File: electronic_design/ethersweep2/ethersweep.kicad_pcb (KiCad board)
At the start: 2 copper layers, 79 x 38 mm, 69 parts, among them J1 AVR-ISP-6, J2 Conn_01x02_Male, J3 Conn_01x04_Female, J4 Conn_01x02_Male, J5 Conn_01x02_Male, J6 HR911105A, J7 Conn_01x06_Female, J8 AVR-ISP-6, J9 Conn_01x06_Male, M1 Stepper_Motor_bipolar, SW1 SW_Push, U1 ENC28J60x-SS, U2 ATmega328-AU, U3 DRV8825PWPR, U4 AMS1117-3.3, U5 AS5600, Y1 Crystal_25MHz, Y2 Crystal_8MHz

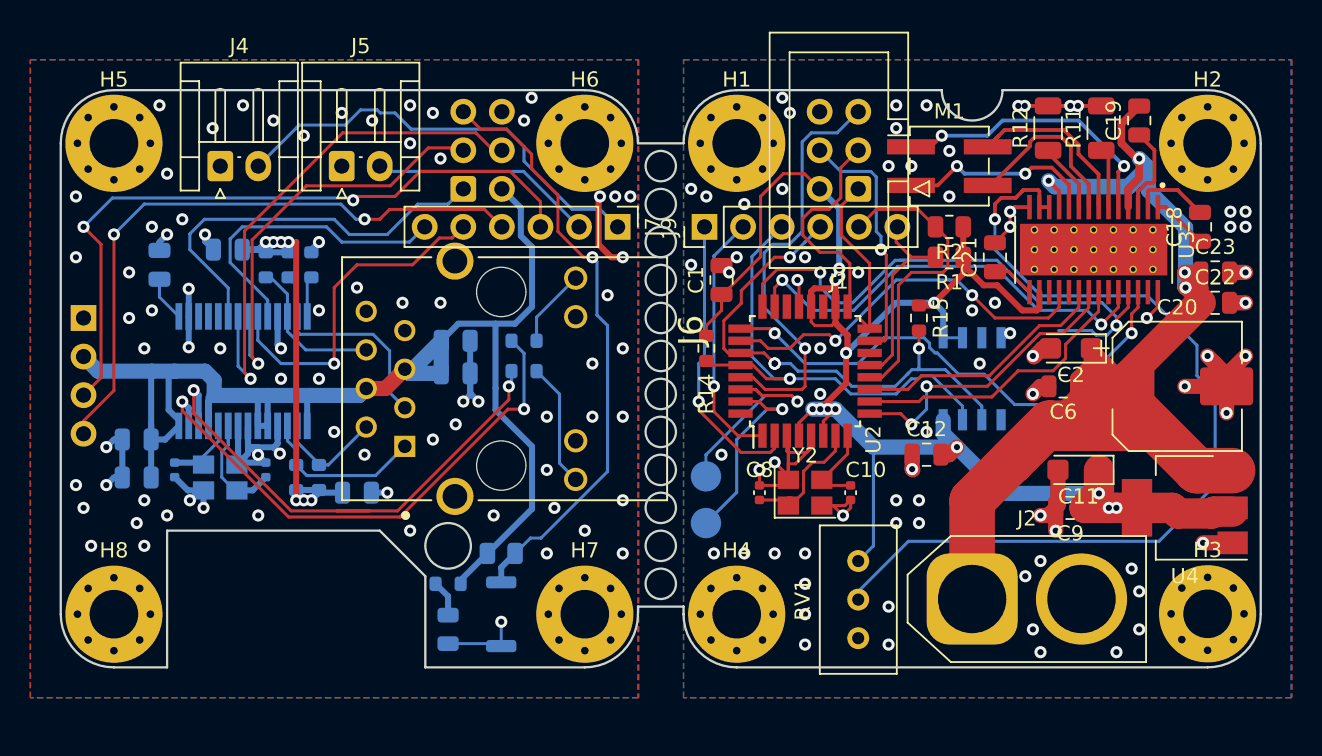
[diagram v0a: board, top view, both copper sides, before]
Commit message: design improvements and error fixes
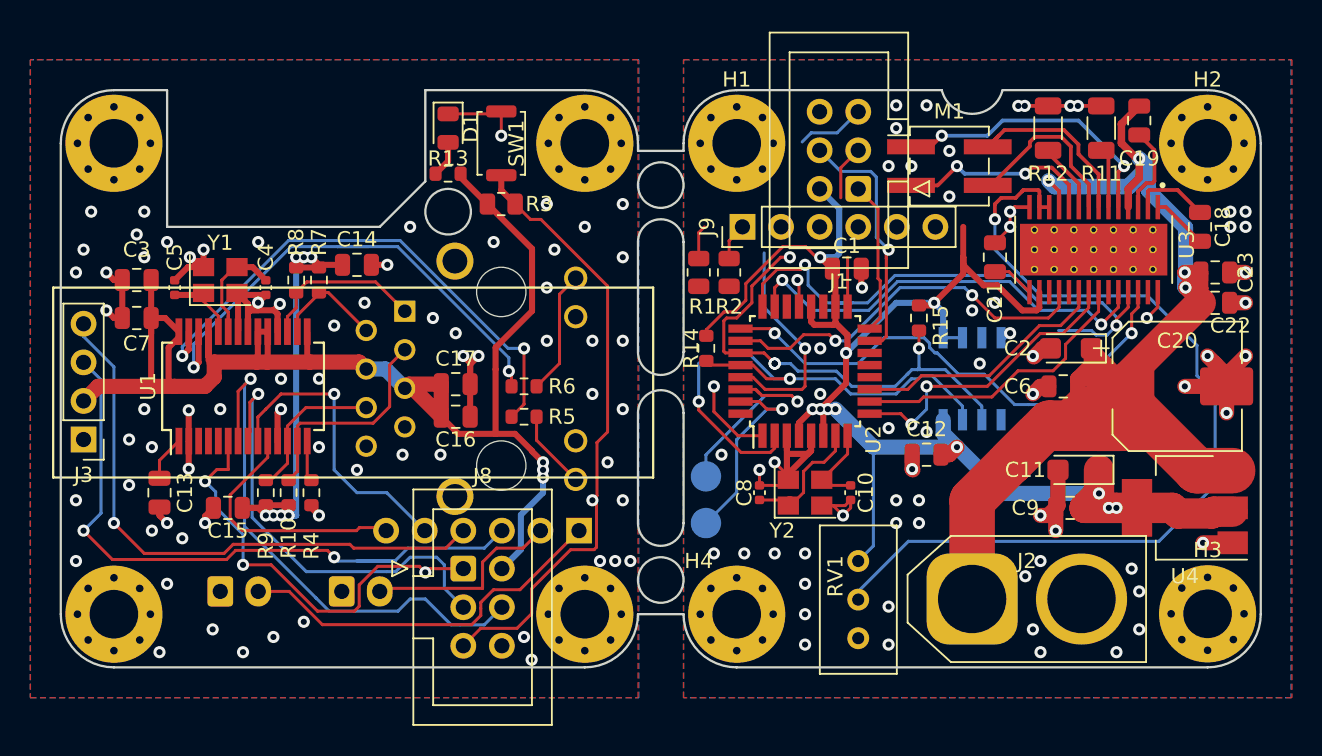
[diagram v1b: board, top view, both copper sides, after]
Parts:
- C13, C14, C15, C16, C17, C3, C4, C5, C7, D1, J3, J8, R10, R13, R3, R4, R5, R6, R7, R8, R9, SW1, U1, Y1: moved to F.Cu
- H5, H6, H7, H8, J4, J5, J6, J7: moved to B.Cu
- moved D1 33.0 mm to (148.0, 83.5), turned to 270 degrees
- moved H5 31.0 mm to (126.0, 115.5)
- moved H6 31.0 mm to (157.0, 115.5)
- moved H7 31.0 mm to (157.0, 84.5)
- moved H8 31.0 mm to (126.0, 84.5)
- moved SW1 31.0 mm to (151.5, 84.5), turned to 90 degrees
- moved J4 28.0 mm to (133.0, 114.0)
- moved J5 28.0 mm to (141.0, 114.0)
- moved R13 27.0 mm to (148.0, 86.5)
- moved J8 25.0 mm to (149.0, 112.5)
- moved R3 23.0 mm to (151.5, 88.5)
- moved J7 20.2 mm to (156.6, 110.0), turned to 90 degrees
- moved C15 17.0 mm to (133.5, 108.5)
- moved R1 16.5 mm to (164.5, 93.0), turned to 90 degrees
- moved C13 15.0 mm to (129.0, 107.5), turned to 270 degrees
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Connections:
- net SLP_ETHERNET renamed Net-(U2-Pad14)
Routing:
- net ENDSTOP: track 34.8 -> 16.2 mm
- net ESTOP: track 41.7 -> 27.3 mm, vias 1 -> 0
- net CS_ETHERNET: track 39.2 -> 25.4 mm
- net RST_ETHERNET: track 39.4 -> 27.6 mm
- net SCL: track 78.7 -> 67.3 mm
- net rst: track 67.6 -> 59.8 mm
- net SCK: track 43.0 -> 37.2 mm
- net SDA: track 76.6 -> 71.1 mm, vias 6 -> 5
- net GND: track 109.2 -> 112.7 mm, vias 149 -> 134
- net +3V3: track 219.5 -> 217.8 mm, vias 13 -> 14
- net M0: track 29.2 -> 28.3 mm
- net M1: track 37.1 -> 37.8 mm
- net MISO: track 38.0 -> 38.4 mm, vias 0 -> 3
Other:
- outline, holes or cut-outs redrawn
- board text added: "VERSION: 2.0.1"
- board text added: "by Neumi 2021-02-03"
